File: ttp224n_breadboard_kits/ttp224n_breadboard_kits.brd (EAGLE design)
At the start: 21.5 x 24.5 mm, 24 parts, among them U1 TTP224N-BSB

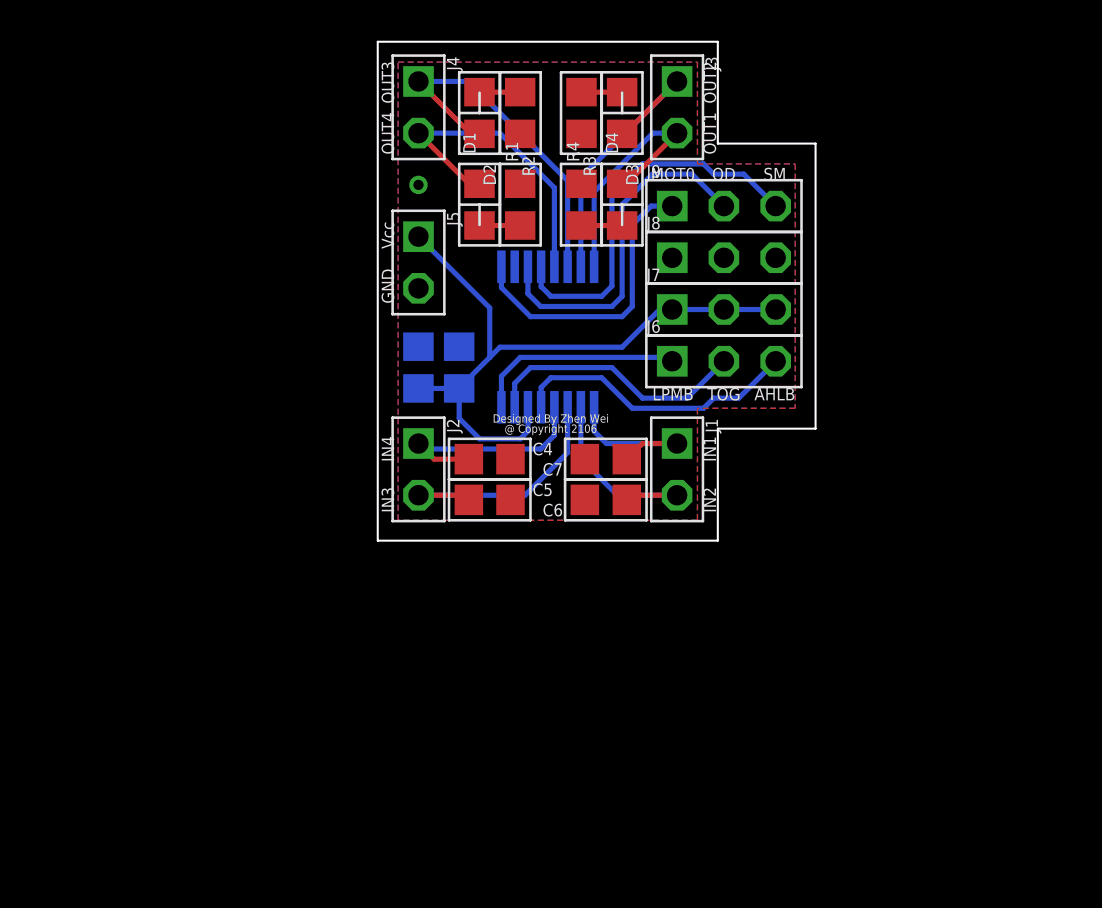
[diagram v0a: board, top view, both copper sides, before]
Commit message: make the change and ttp224n_breadboard_kits is ready to go
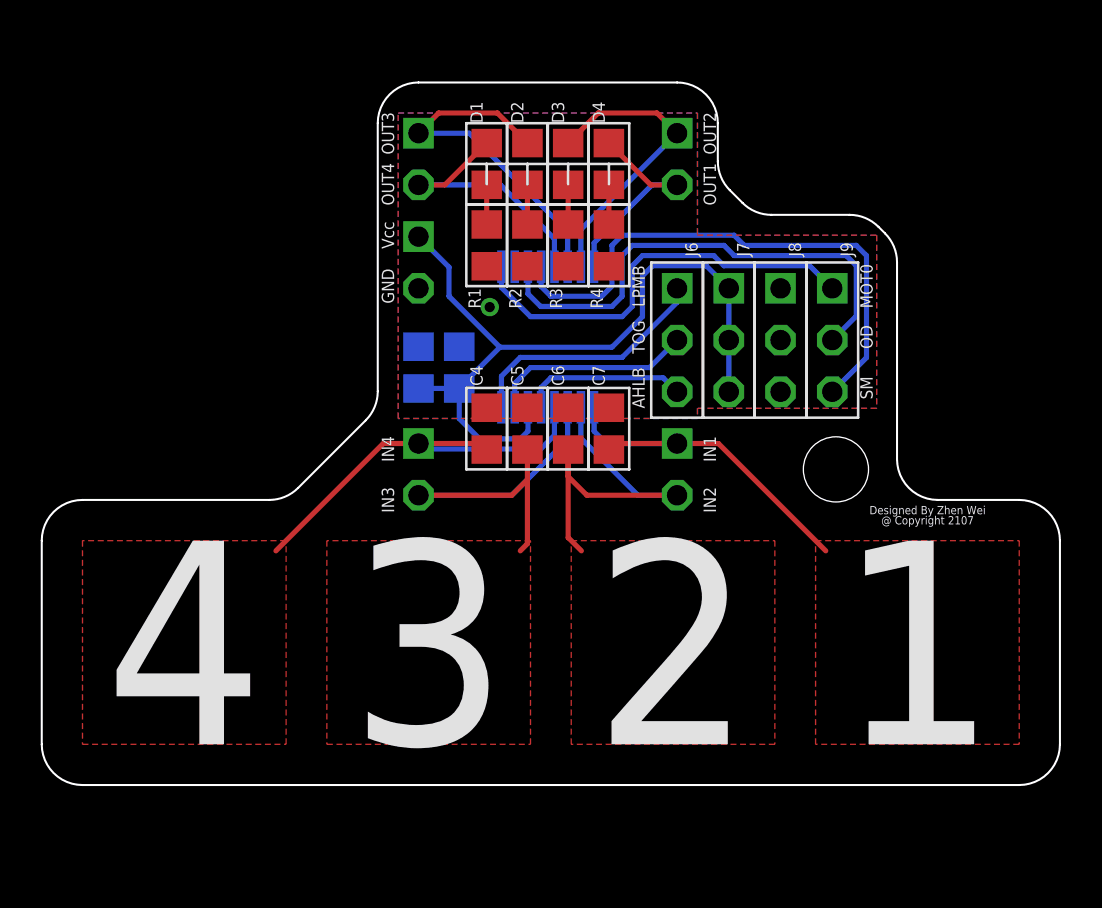
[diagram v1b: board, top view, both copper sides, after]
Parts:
- moved J9 8.46 mm to (22.3, 9.85), turned to 270 degrees
- moved R3 6.53 mm to (9.35, 14.5)
- moved R2 6.51 mm to (7.35, 14.5)
- moved J8 4.90 mm to (19.8, 9.85), turned to 270 degrees
- moved C5 3.96 mm to (7.35, 5.50), turned to 90 degrees
- moved C6 3.96 mm to (9.35, 5.50), turned to 90 degrees
- moved D3 3.64 mm to (9.35, 18.5), turned to 90 degrees
- moved D2 3.43 mm to (7.35, 18.5), turned to 90 degrees
- moved R1 2.59 mm to (5.35, 14.5), turned to 270 degrees
- moved J3 2.54 mm to (14.7, 18.7), flipped to the bottom
- moved J4 2.54 mm to (2.00, 18.7), flipped to the bottom
- moved J6 2.52 mm to (14.7, 9.85), turned to 270 degrees
- moved R4 2.41 mm to (11.3, 14.5), turned to 270 degrees
- moved D4 2.10 mm to (11.3, 18.5)
- moved D1 2.03 mm to (5.35, 18.5)
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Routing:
- net IN1: track 8.29 -> 18.5 mm
- net IN4: track 11.2 -> 21.1 mm
- net IN2: track 10.6 -> 19.7 mm
- net SM: track 18.9 -> 27.4 mm
- net IN3: track 13.0 -> 20.8 mm
- net OD: track 17.2 -> 24.7 mm
- net MOT0: track 14.6 -> 20.9 mm
- net AHLB: track 14.3 -> 8.13 mm
- net +3V3: track 33.1 -> 38.1 mm
- net TOG: track 13.1 -> 10.0 mm
- net OUT4: track 15.8 -> 13.3 mm
- net OUT1: track 12.7 -> 10.6 mm
- net LPMB: track 10.4 -> 12.3 mm
- added copper zone on layer 1, net IN1
- added copper zone on layer 1, net IN2
- added copper zone on layer 1, net IN3
- added copper zone on layer 1, net IN4
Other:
- board size 21.5 x 24.5 mm -> 50 x 34.5 mm
- board text added: "1"
- board text added: "2"
- board text added: "3"
- board text added: "4"
- board text added: "@ Copyright 2107"
- board text removed: "@ Copyright 2106"
